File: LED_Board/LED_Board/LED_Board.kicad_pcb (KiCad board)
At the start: 2 copper layers, 8 parts, among them J1 Conn_01x04

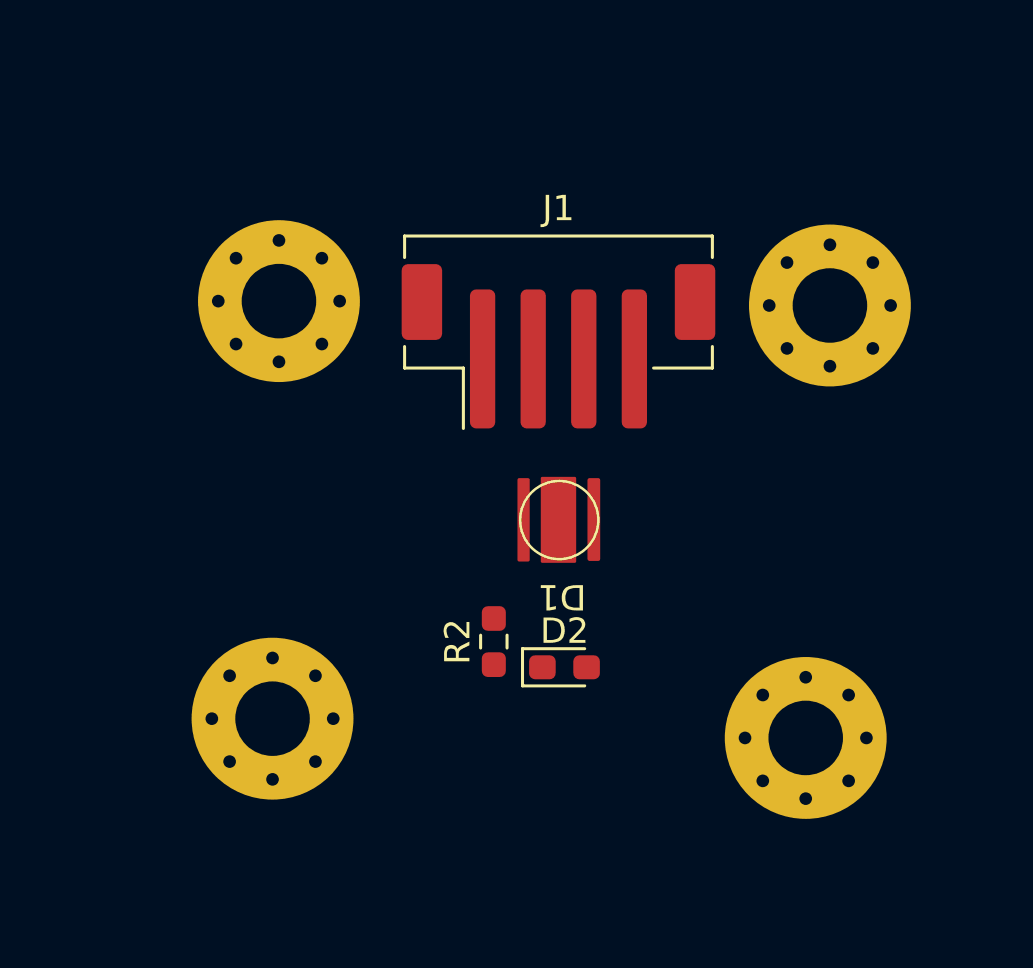
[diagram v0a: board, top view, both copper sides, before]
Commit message: Finalized Initial Layout
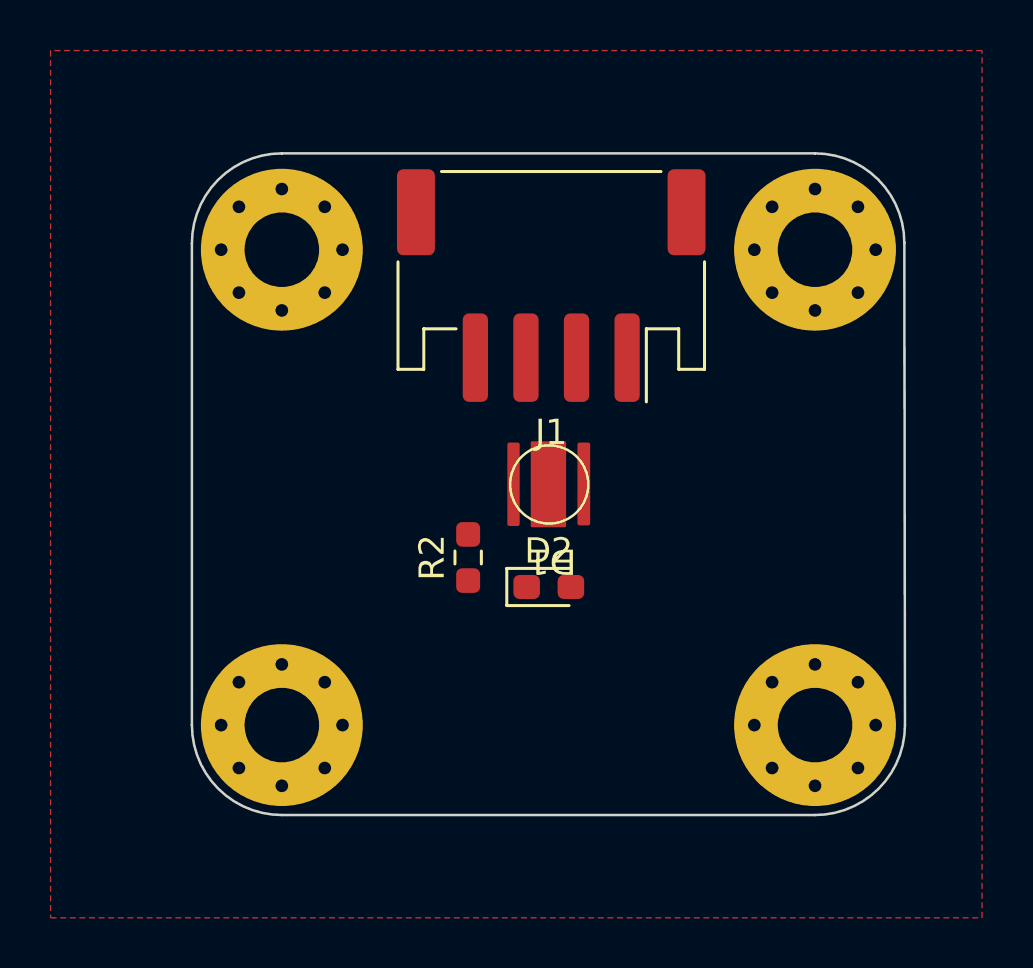
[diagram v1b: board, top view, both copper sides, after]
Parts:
- J1: footprint Connector_JST:JST_PH_B4B-PH-SM4-TB_1x04-1MP_P2.00mm_Vertical -> Connector_JST:JST_PH_S4B-PH-SM4-TB_1x04-1MP_P2.00mm_Horizontal
- moved R2 3.48 mm to (167.6, 102.6)
- moved D2 3.24 mm to (170.8, 103.8)
- moved J1 2.42 mm to (170.9, 91.8), turned to 180 degrees
- moved H2 2.28 mm to (181.4, 90.4)
- moved H1 2.04 mm to (160.3, 90.4)
- moved D1 1.46 mm to (170.8, 99.7)
- moved H4 0.63 mm to (181.4, 109.2)
- moved H3 0.45 mm to (160.3, 109.2)
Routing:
- added copper zone on F.Cu, net GND
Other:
- board outline added: 28.2 x 26.2 mm
